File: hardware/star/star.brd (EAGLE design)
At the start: 139.4 x 187.9 mm, 160 parts, among them IC1 MAX481CSA, IC2 74HCT08D, IC22 LD117AS12TR, IC3 74HCT08D, IC4 7404D, IC8 MAX481CSA, K1 T90-12VDC-TL-A, K2 T90-12VDC-TL-A, K3 T90-12VDC-TL-A, K5 AQG22110, K6 AQG22110, Q1 35A/25V/8.5mΩ, Q2 35A/25V/8.5mΩ, Q3 35A/25V/8.5mΩ, Q4 35A/25V/8.5mΩ, U1 TCLT1600, U2 ADXL343BCCZ-RL7, U3 TMP102AIDRLR, U4 SN74LVC1G17DCK, U5 SN74LVC1G17DCK, U6 SN74LVC1G17DCK, U7 SN74LVC1G17DCK, X1 MKDSN1,5/2-5,08

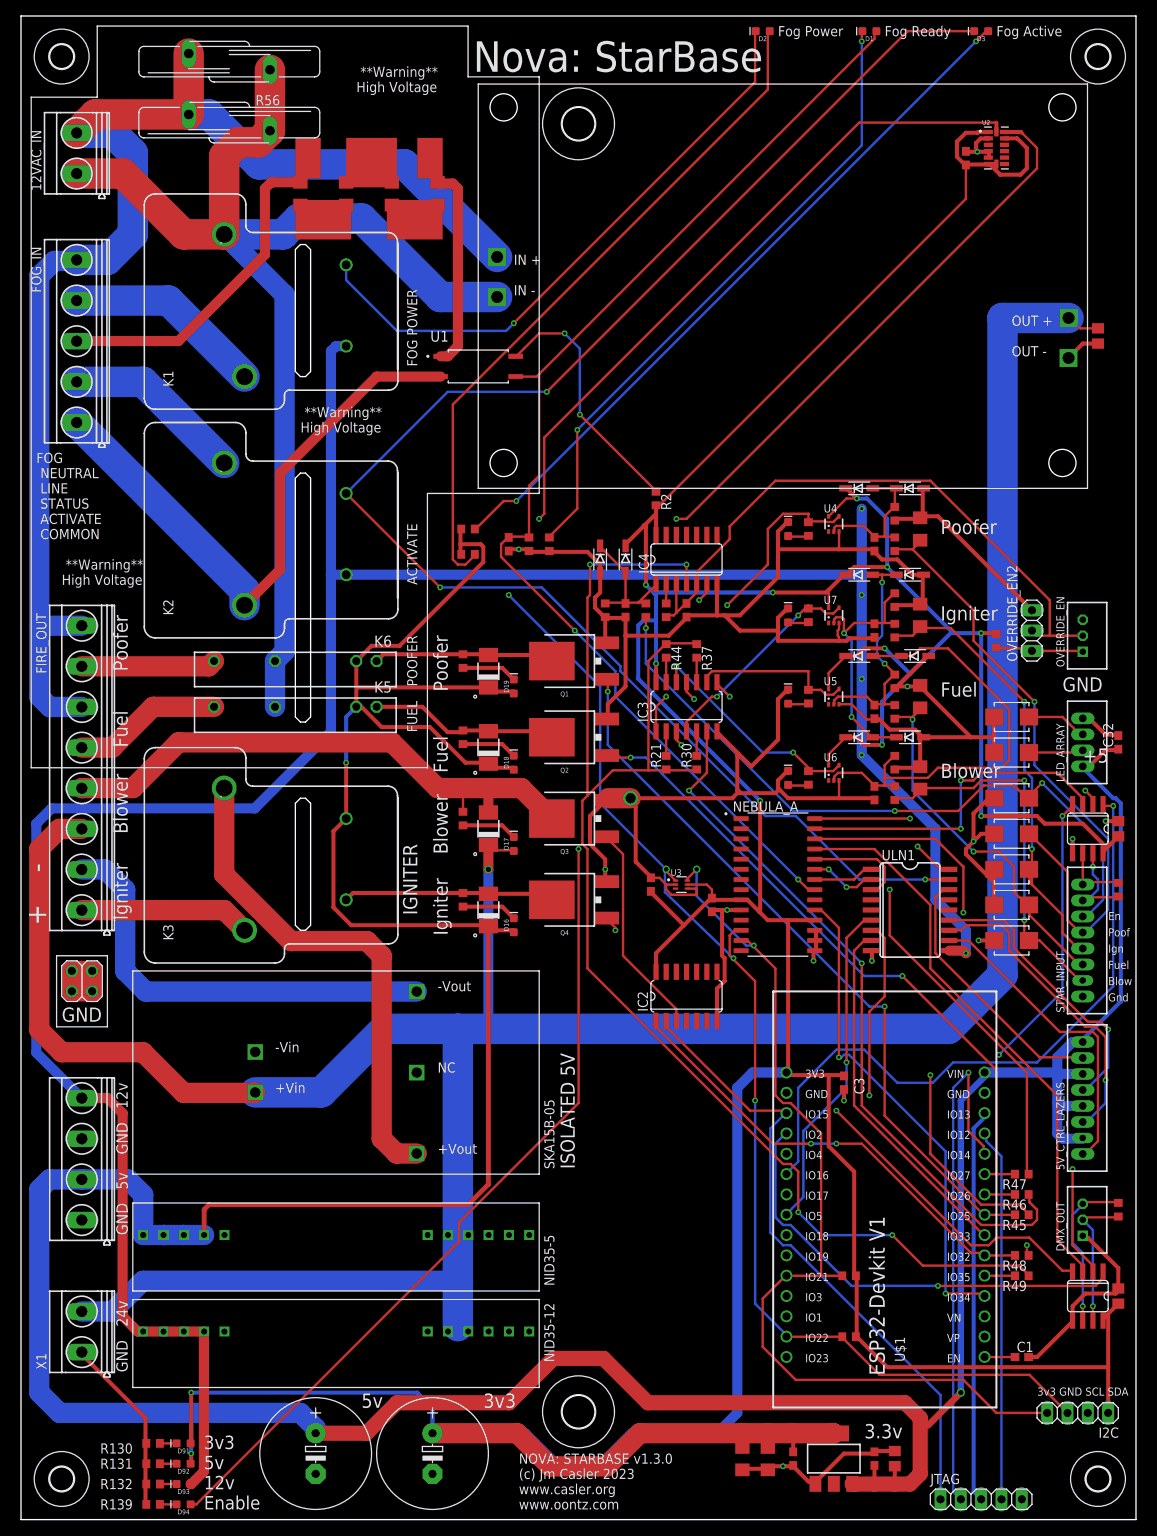
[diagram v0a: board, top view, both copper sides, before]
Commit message: Initial code for starbase
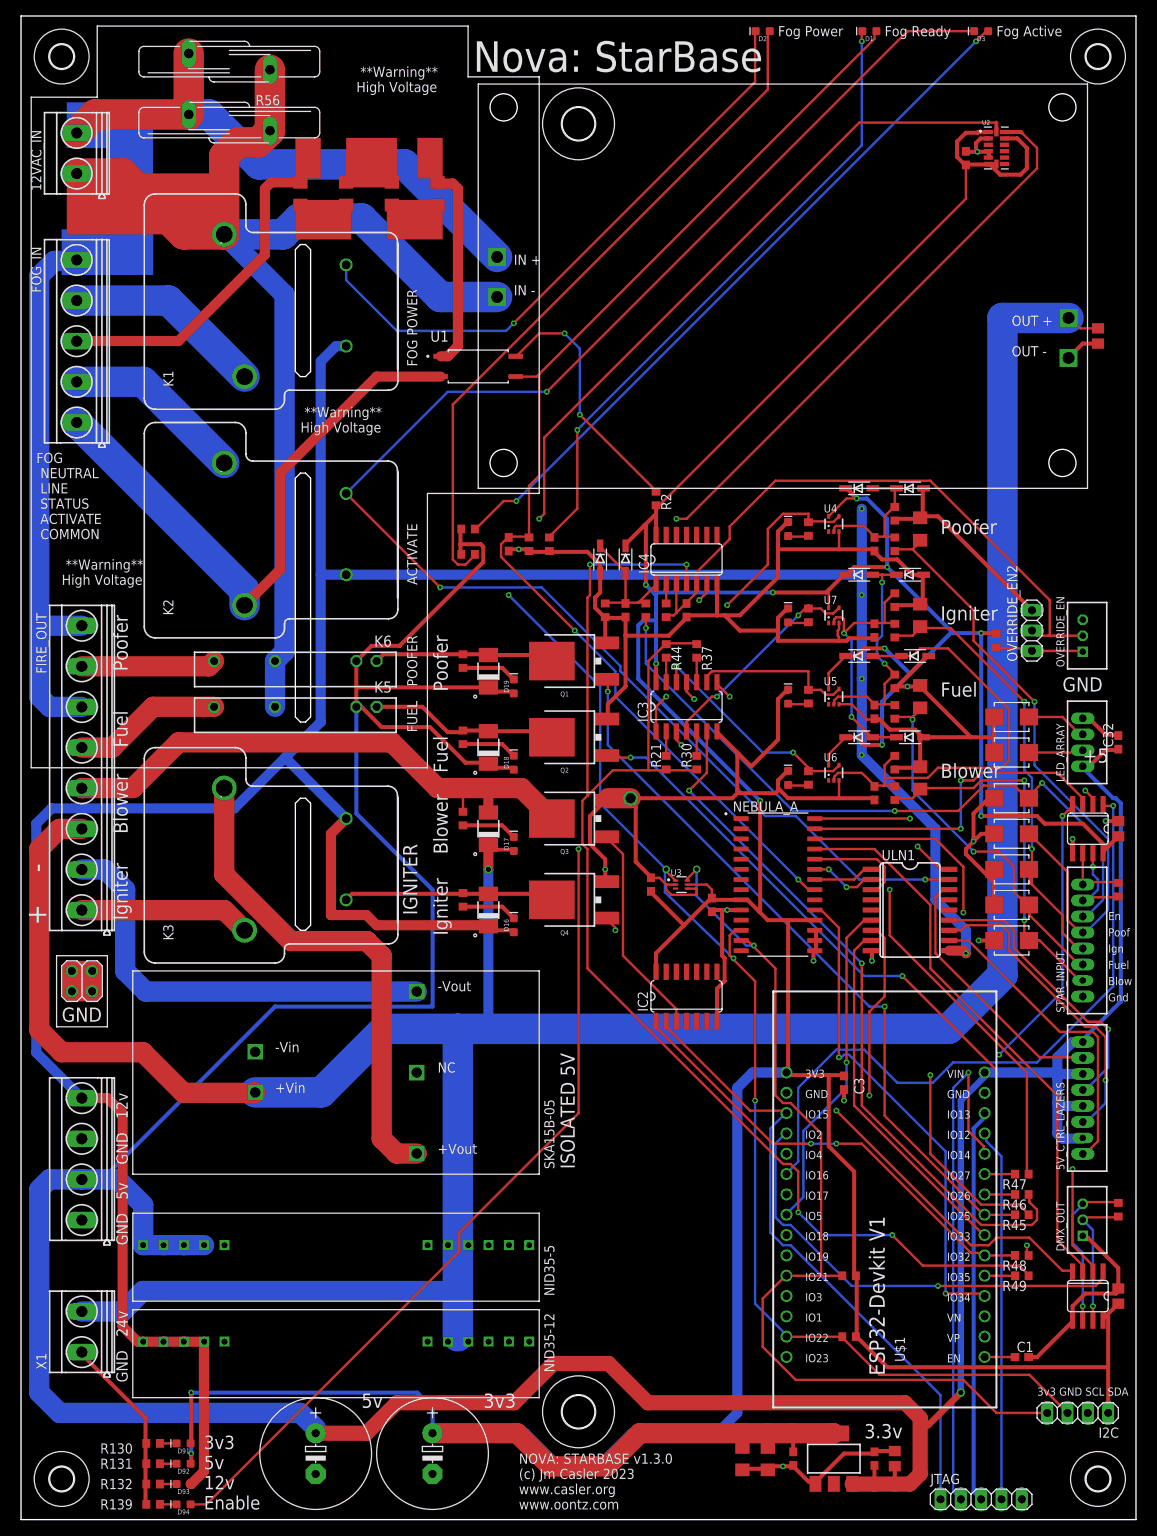
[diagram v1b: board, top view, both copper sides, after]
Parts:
- R15: value R_1K_0603 -> R_2K_0603
- moved NID35-12 1.27 mm to (14.0, 15.2)
- moved NID35-5 1.27 mm to (14.0, 27.3)
- renumbered R63 to R15
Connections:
- net +12V: now also D15.C, D16.A, K3.1
- net +5V: no longer D15.C, D16.A, K3.1
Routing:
- net +12V: track 319.8 -> 367.3 mm
- net +5V: track 525.7 -> 494.2 mm, vias 3 -> 2
- net +24V: track 372.2 -> 376.4 mm
- net EN_STATUS: track 142.2 -> 142.9 mm
